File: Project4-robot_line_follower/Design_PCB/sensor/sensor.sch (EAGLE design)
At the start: 57 parts

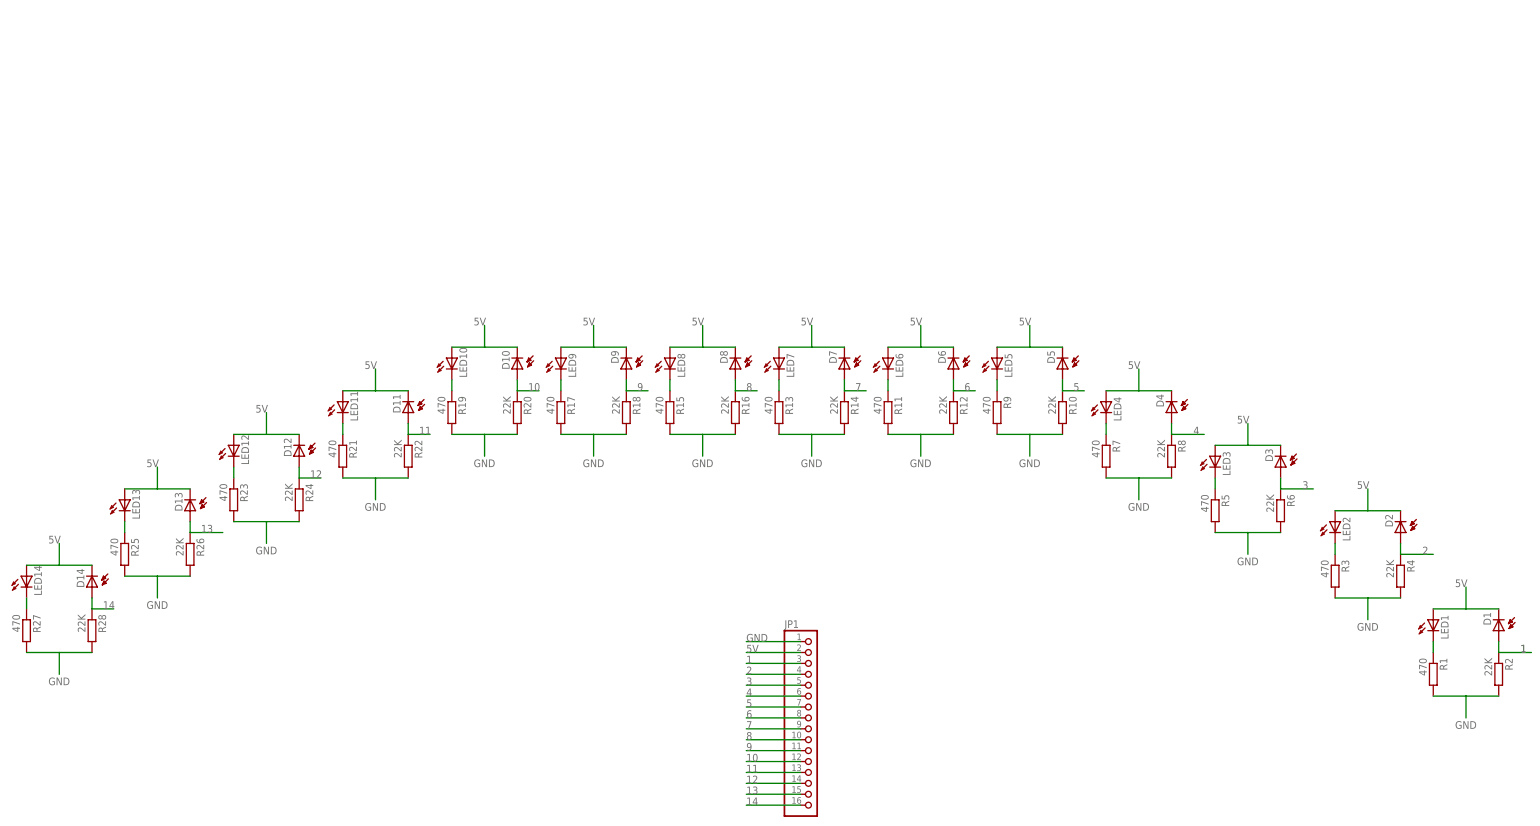
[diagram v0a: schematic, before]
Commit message: rename file
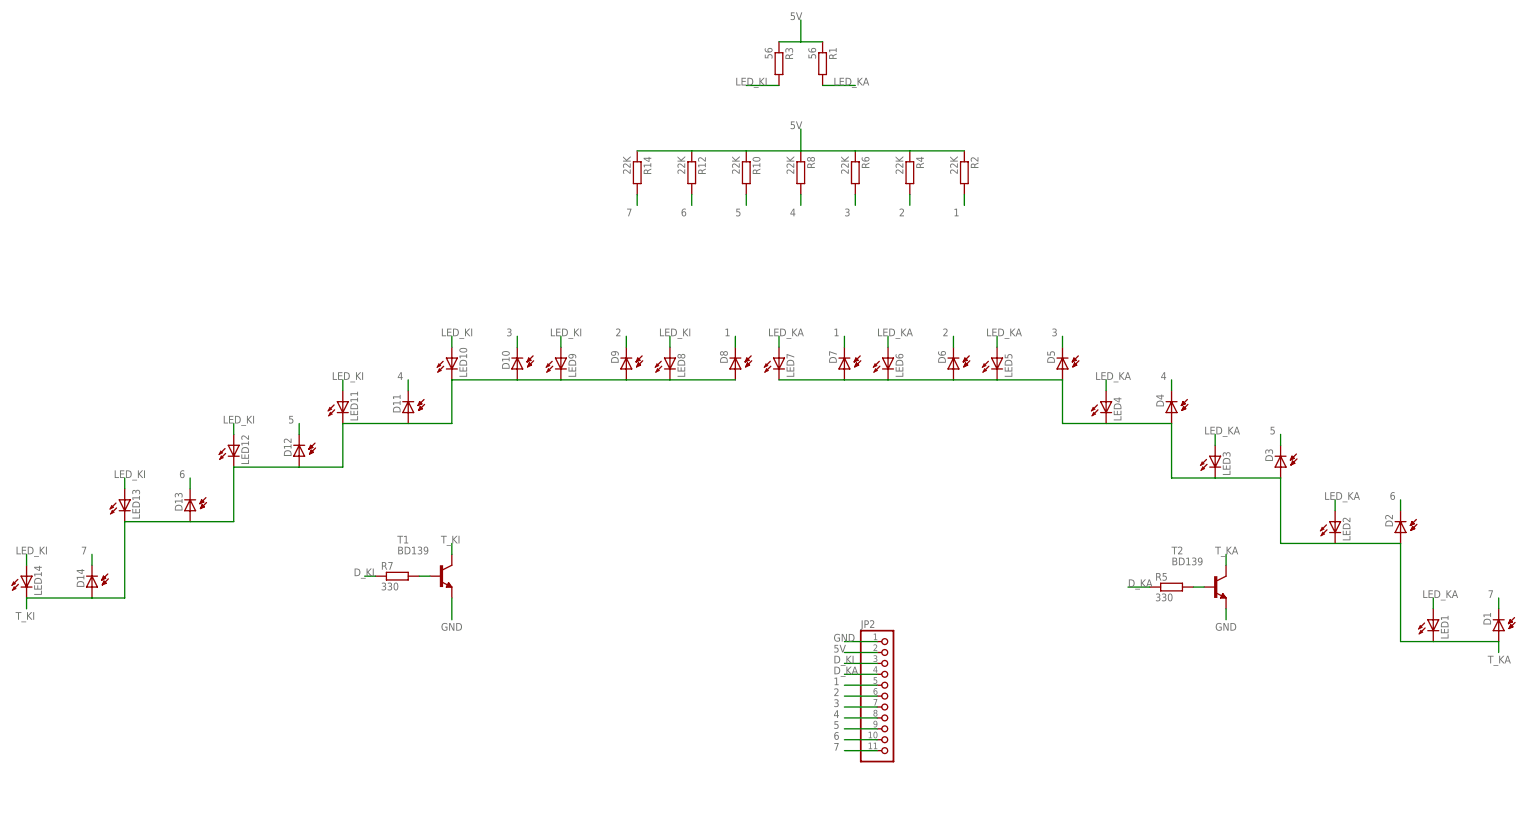
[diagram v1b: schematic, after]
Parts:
- removed JP1: (no value), pinhead:PINHD-1X16
- removed R11, R13, R15, R17, R19, R21, R23, R25, R27, R9: 470, rcl:R-EU_0207/7
- removed R16, R18, R20, R22, R24, R26, R28: 22K, rcl:R-EU_0207/7
- added JP2: (no value), pinhead:PINHD-1X11
- added T1, T2: BD139, transistor:BD139
- R1, R3: value 470 -> 56
- R5, R7: value 470 -> 330
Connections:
- removed net 10: D10.A, JP1.12, R20.1
- removed net 11: D11.A, JP1.13, R22.1
- removed net 12: D12.A, JP1.14, R24.1
- removed net 13: D13.A, JP1.15, R26.1
- removed net 14: D14.A, JP1.16, R28.1
- removed net 8: D8.A, JP1.10, R16.1
- removed net 9: D9.A, JP1.11, R18.1
- removed net N$11: LED6.C, R11.1
- removed net N$13: LED7.C, R13.1
- removed net N$15: LED8.C, R15.1
- removed net N$17: LED9.C, R17.1
- removed net N$19: LED10.C, R19.1
- removed net N$21: LED11.C, R21.1
- removed net N$23: LED12.C, R23.1
- removed net N$25: LED13.C, R25.1
- removed net N$27: LED14.C, R27.1
- removed net N$3: LED2.C, R3.1
- removed net N$5: LED3.C, R5.1
- removed net N$7: LED4.C, R7.1
- removed net N$9: LED5.C, R9.1
- new net D_KA: JP2.4, R5.1
- new net D_KI: JP2.3, R7.1
- new net LED_KA: LED1.A, LED2.A, LED3.A, LED4.A, LED5.A, LED6.A, LED7.A, R1.2
- new net LED_KI: LED10.A, LED11.A, LED12.A, LED13.A, LED14.A, LED8.A, LED9.A, R3.2
- new net N$2: R5.2, T2.B
- new net T_KA: D1.A, D2.A, D3.A, D4.A, D5.A, D6.A, D7.A, LED1.C, LED2.C, LED3.C, LED4.C, LED5.C, LED6.C, LED7.C, T2.C
- new net T_KI: D10.A, D11.A, D12.A, D13.A, D14.A, D8.A, D9.A, LED10.C, LED11.C, LED12.C, LED13.C, LED14.C, LED8.C, LED9.C, T1.C
- net 1: now also D7.C, D8.C, JP2.5, R2.2; no longer D1.A, JP1.3, R2.1
- net 2: now also D6.C, D9.C, JP2.6, R4.2; no longer D2.A, JP1.4, R4.1
- net 3: now also D10.C, D5.C, JP2.7, R6.2; no longer D3.A, JP1.5, R6.1
- net 4: now also D11.C, D4.C, JP2.8, R8.2; no longer D4.A, JP1.6, R8.1
- net 5: now also D12.C, D3.C, JP2.9, R10.2; no longer D5.A, JP1.7, R10.1
- net 5V: now also JP2.2, R1.1, R10.1, R12.1, R14.1, R2.1, R3.1, R4.1, R6.1, R8.1; no longer D1.C, D10.C, D11.C, D12.C, D13.C, D14.C, D2.C, D3.C, D4.C, D5.C, D6.C, D7.C, D8.C, D9.C, JP1.2, LED1.A, LED10.A, LED11.A, LED12.A, LED13.A, LED14.A, LED2.A, LED3.A, LED4.A, LED5.A, LED6.A, LED7.A, LED8.A, LED9.A
- net 6: now also D13.C, D2.C, JP2.10, R12.2; no longer D6.A, JP1.8, R12.1
- net 7: now also D1.C, D14.C, JP2.11, R14.2; no longer D7.A, JP1.9, R14.1
- net GND: now also JP2.1, T1.E, T2.E; no longer JP1.1, R1.2, R10.2, R11.2, R12.2, R13.2, R14.2, R15.2, R16.2, R17.2, R18.2, R19.2, R2.2, R20.2, R21.2, R22.2, R23.2, R24.2, R25.2, R26.2, R27.2, R28.2, R3.2, R4.2, R5.2, R6.2, R7.2, R8.2, R9.2
- net N$1: now also R7.2, T1.B; no longer LED1.C, R1.1
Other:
- moved on the sheet: R1, R10, R12, R14, R2, R3, R4, R5, R6, R7, R8
